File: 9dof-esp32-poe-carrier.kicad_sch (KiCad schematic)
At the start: 6 parts, among them J1 Input Power, J2 Stemma QT, J3 UEXT_Slave, J4 WS2811_strand, J5 USB_A, U1 AMS1117-5.0

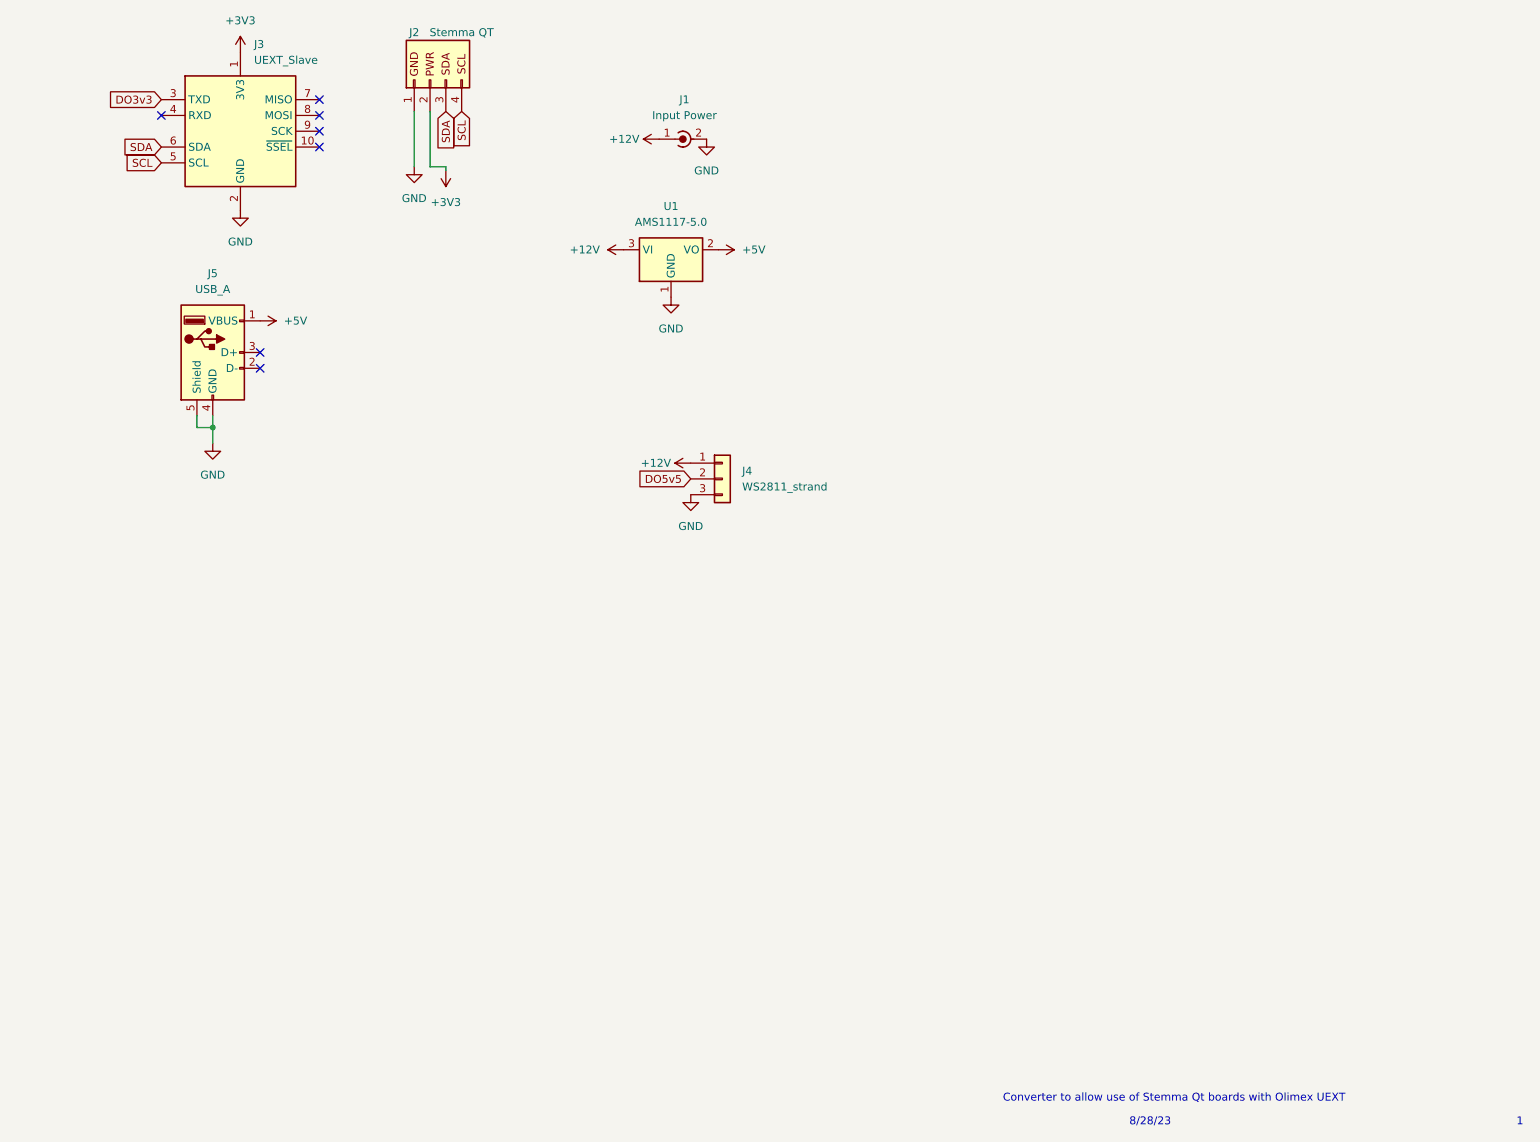
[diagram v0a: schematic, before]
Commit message: Updated redone schematic.
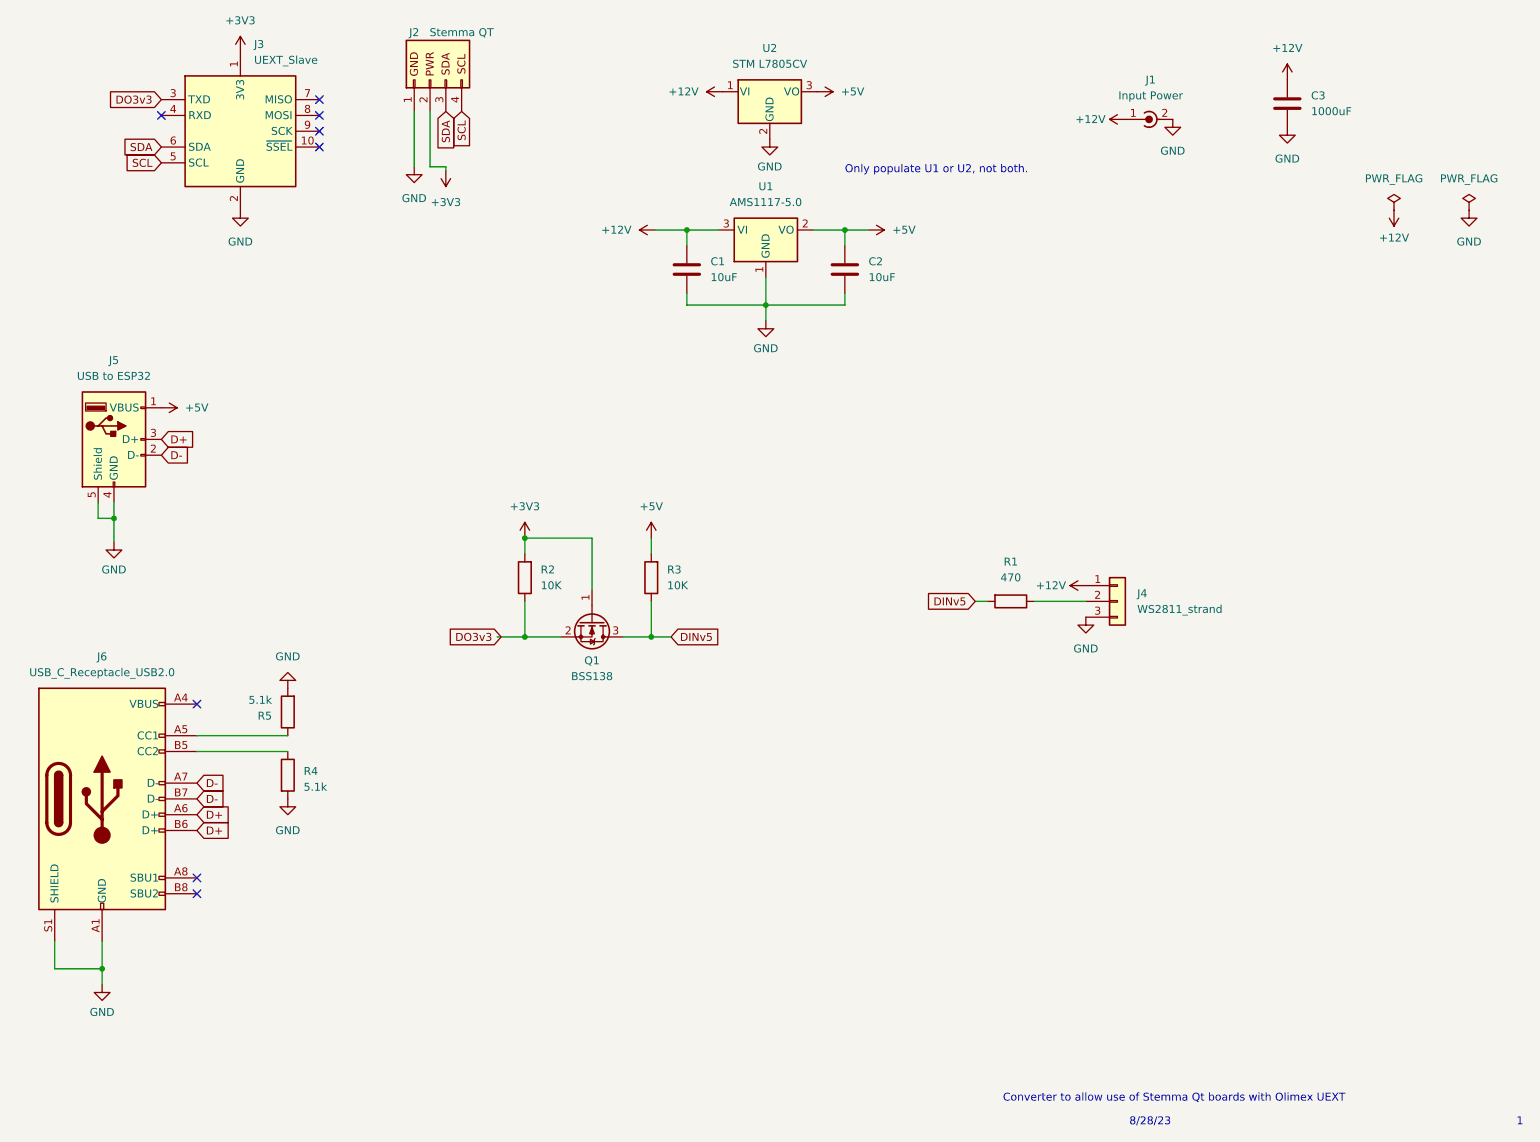
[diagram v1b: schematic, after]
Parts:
- added C1, C2: 10uF, Capacitor_SMD:C_0402_1005Metric_Pad0.74x0.62mm_HandSolder, symbol Device:C
- added C3: 1000uF, EasyEDA_Footprints:CAP-SMD_BD10.0-L10.3-W10.3-FD, symbol Device:C
- added J6: USB_C_Receptacle_USB2.0, EasyEDA_Footprints:USB-C_SMD-TYPE-C-31-M-12, symbol Connector:USB_C_Receptacle_USB2.0
- added Q1: BSS138, EasyEDA_Footprints:SOT-23-3_L2.9-W1.3-P1.90-LS2.4-BR, symbol Transistor_FET:BSS138
- added R1: 470, Resistor_SMD:R_0402_1005Metric_Pad0.72x0.64mm_HandSolder, symbol Device:R
- added R2, R3: 10K, Resistor_SMD:R_0402_1005Metric_Pad0.72x0.64mm_HandSolder, symbol Device:R
- added R4, R5: 5.1k, Resistor_SMD:R_0402_1005Metric, symbol Device:R
- added U2: STM L7805CV, Package_TO_SOT_THT:TO-220-3_Vertical, symbol Regulator_Linear:LM7805_TO220
- J1: footprint Connector_BarrelJack:BarrelJack_Horizontal -> EasyEDA_Footprints:DC-IN-TH_DC005-T; LCSC (none) -> C431532
- J2: footprint Connector_JST:JST_SH_SM04B-SRSS-TB_1x04-1MP_P1.00mm_Horizontal -> EasyEDA_Footprints:CONN-SMD_4P-P1.00_SM04B-SRSS-TB-LF-SN
- J3: footprint Connector_PinHeader_2.54mm:PinHeader_2x05_P2.54mm_Vertical -> Library:UEXT_SLAVE_BACKSIDE
- J5: value USB_A -> USB to ESP32; footprint Connector_USB:USB_A_Receptacle_GCT_USB1046 -> (none)
- U1: footprint Package_TO_SOT_SMD:SOT-223-3_TabPin2 -> EasyEDA_Footprints:SOT-223-3_L6.7-W3.7-P2.30-LS7.0-BR; LSCS C6187 -> C917153
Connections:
- net +12V: now also C1.1, C3.1, U2.1 (VI)
- net +3V3: now also Q1.1 (G), R2.2
- net +5V: now also C2.1, R3.2, U2.3 (VO)
- net DO3v3: now also Q1.2 (S), R2.1
- net GND: now also C1.2, C2.2, C3.2, J6.A1 (GND), J6.A12 (GND), J6.B1 (GND), J6.B12 (GND), J6.S1 (SHIELD), R4.2, R5.2, U2.2 (GND)
- net D-: now reaches J5.2 (D-)
- net D-: now also J6.A7 (D-), J6.B7 (D-)
- net D+: now reaches J5.3 (D+)
- net D+: now also J6.A6 (D+), J6.B6 (D+)
- net DO5v5: no longer names the net of J4.2 (Pin_2)
- net DO5v5: now also R1.1
- new net: J6.A5 (CC1), R5.1
- new net: J6.A4 (VBUS), J6.A9 (VBUS), J6.B4 (VBUS), J6.B9 (VBUS)
- new net: J6.B5 (CC2), R4.1
- new net DINv5: Q1.3 (D), R1.2, R3.1
- no-connect marks 7 -> 8
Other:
- note added: "Only populate U1 or U2, not both."
- moved on the sheet: J1, J4, U1

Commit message: Fiddle with parts, add via stiching, add silkscreen labels.
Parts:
- C1, C2: LCSC (none) -> C15525
- J4: LCSC (none) -> C49257
- J5: footprint (none) -> Connector_PinHeader_2.54mm:PinHeader_1x05_P2.54mm_Vertical; LCSC (none) -> C492404
- R1: LCSC (none) -> C25117
- R2, R3: LCSC (none) -> C25744
- R4, R5: footprint Resistor_SMD:R_0402_1005Metric -> Resistor_SMD:R_0402_1005Metric_Pad0.72x0.64mm_HandSolder; LCSC (none) -> C25905
- U1: LCSC (none) -> C917153; LSCS C917153 -> (none)
- U2: Fitted (none) -> N
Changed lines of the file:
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@@
+      (effects (font (size 1.27 1.27)) hide)
+    )
+    (property "LCSC" "C49257" (at 205.105 109.855 0)
       (effects (font (size 1.27 1.27)) hide)
     )
@@
       (effects (font (size 1.27 1.27)) hide)
     )
+    (property "LCSC" "C25744" (at 130.175 106.045 0)
+      (effects (font (size 1.27 1.27)) hide)
+    )
     (pin "1")
     (pin "2")
@@
       (effects (font (size 1.27 1.27)))
     )
-    (property "Footprint" "" (at 47.625 85.09 0)
+    (property "Footprint" "Connector_PinHeader_2.54mm:PinHeader_1x05_P2.54mm_Vertical" (at 47.625 85.09 0)
       (effects (font (size 1.27 1.27)) hide)
     )
     (property "Datasheet" " ~" (at 47.625 85.09 0)
+      (effects (font (size 1.27 1.27)) hide)
+    )
+    (property "LCSC" "C492404" (at 43.815 83.82 0)
       (effects (font (size 1.27 1.27)) hide)
     )
@@
     )
     (property "Datasheet" "~" (at 187.96 109.855 0)
+      (effects (font (size 1.27 1.27)) hide)
+    )
+    (property "LCSC" "C25117" (at 187.96 109.855 0)
       (effects (font (size 1.27 1.27)) hide)
     )
@@
       (effects (font (size 1.27 1.27)) (justify left))
     )
-    (property "Footprint" "Resistor_SMD:R_0402_1005Metric" (at 73.533 127.635 90)
+    (property "Footprint" "Resistor_SMD:R_0402_1005Metric_Pad0.72x0.64mm_HandSolder" (at 73.533 127.635 90)
       (effects (font (size 1.27 1.27)) hide)
     )
     (property "Datasheet" "~" (at 71.755 127.635 0)
+      (effects (font (size 1.27 1.27)) hide)
+    )
+    (property "LCSC" "C25905" (at 71.755 127.635 0)
       (effects (font (size 1.27 1.27)) hide)
     )
@@
     )
     (property "Datasheet" "~" (at 135.89 56.515 0)
+      (effects (font (size 1.27 1.27)) hide)
+    )
+    (property "LCSC" "C15525" (at 135.89 56.515 0)
       (effects (font (size 1.27 1.27)) hide)
     )
@@
       (effects (font (size 1.27 1.27)) hide)
     )
+    (property "LCSC" "C15525" (at 161.29 56.515 0)
+      (effects (font (size 1.27 1.27)) hide)
+    )
     (pin "1")
     (pin "2")
@@
       (effects (font (size 1.27 1.27)) (justify left))
     )
-    (property "Footprint" "Resistor_SMD:R_0402_1005Metric" (at 69.977 137.795 90)
+    (property "Footprint" "Resistor_SMD:R_0402_1005Metric_Pad0.72x0.64mm_HandSolder" (at 69.977 137.795 90)
       (effects (font (size 1.27 1.27)) hide)
     )
     (property "Datasheet" "~" (at 71.755 137.795 0)
+      (effects (font (size 1.27 1.27)) hide)
+    )
+    (property "LCSC" "C25905" (at 71.755 137.795 0)
       (effects (font (size 1.27 1.27)) hide)
     )
@@
       (effects (font (size 1.27 1.27)) hide)
     )
+    (property "LCSC" "C25744" (at 109.855 106.045 0)
+      (effects (font (size 1.27 1.27)) hide)
+    )
     (pin "1")
     (pin "2")
@@
       (effects (font (size 1.27 1.27)) hide)
     )
-    (property "LSCS" "C917153" (at 148.59 50.165 0)
+    (property "LSCS" "" (at 148.59 50.165 0)
+      (effects (font (size 1.27 1.27)) hide)
+    )
+    (property "LCSC" "C917153" (at 148.59 50.165 0)
       (effects (font (size 1.27 1.27)) hide)
     )
@@
       (effects (font (size 1.27 1.27)) hide)
     )
+    (property "Fitted" "N" (at 149.225 27.94 0)
+      (effects (font (size 1.27 1.27)) hide)
+    )
